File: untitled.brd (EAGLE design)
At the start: 59.4 x 57.8 mm, 25 parts

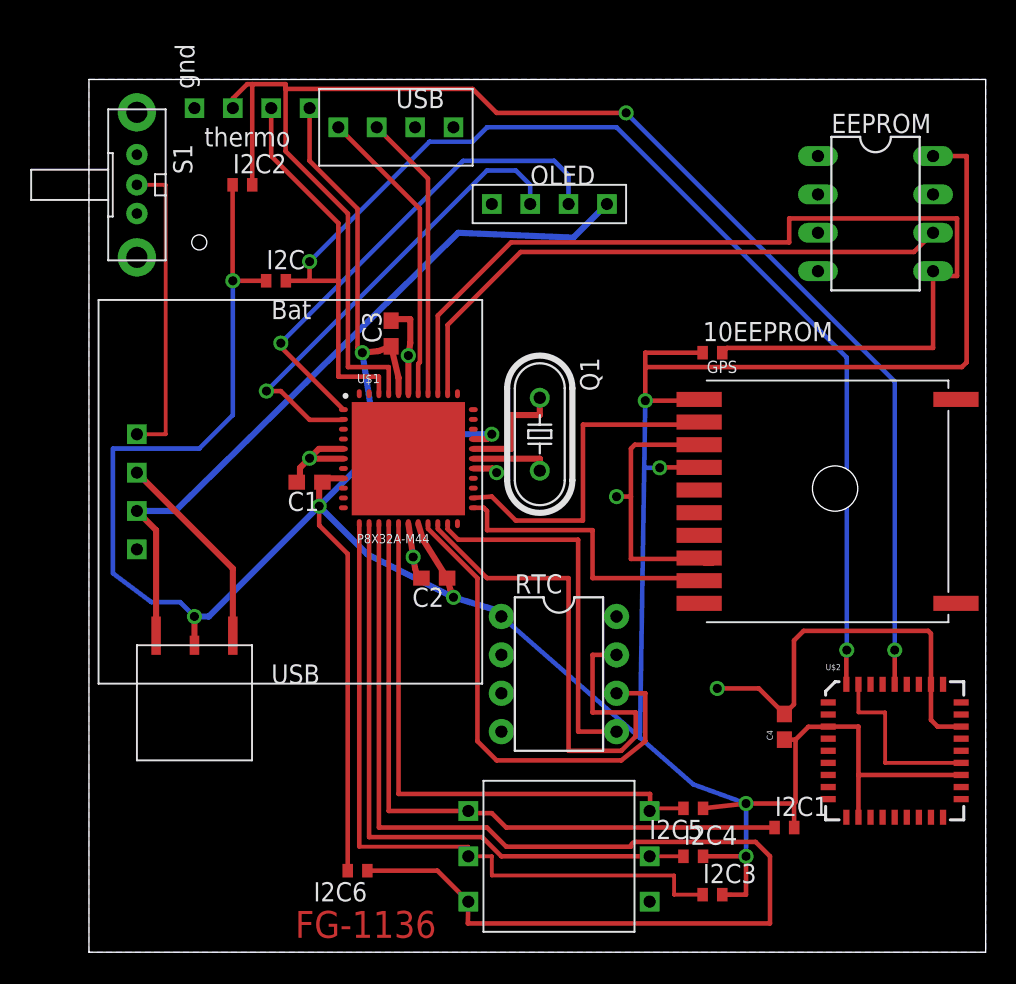
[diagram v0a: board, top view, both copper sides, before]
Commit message: cleaned
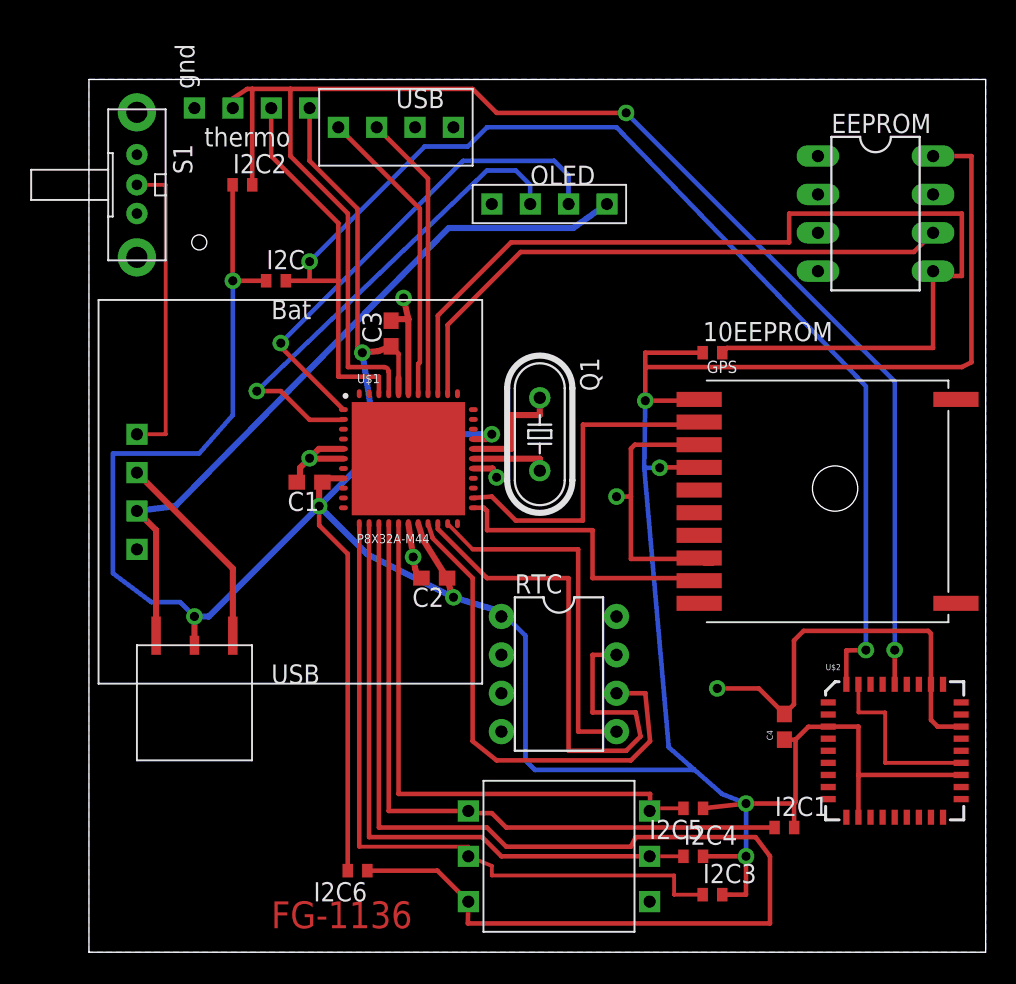
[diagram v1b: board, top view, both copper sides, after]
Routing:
- net +3V3: track 280.7 -> 289.7 mm
- net SDA: track 95.4 -> 97.0 mm
- net GND: track 78.5 -> 80.1 mm
- net N$18: track 67.8 -> 69.1 mm
- net SCL: track 104.5 -> 103.3 mm
- net N$10: track 31.1 -> 32.2 mm
- net N$5: track 24.5 -> 24.0 mm
- net N$17: track 47.3 -> 46.8 mm
- net N$15: track 80.5 -> 81.0 mm
